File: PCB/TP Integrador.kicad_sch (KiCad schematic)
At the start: 37 parts, among them Q1 BC547C, Q10 BC547C, Q11 BC547C, Q2 2SB631, Q3 BC547, Q4 BC547C, Q5 BC557C, Q6 BC557C, Q9 BC547C, U1 TL431D

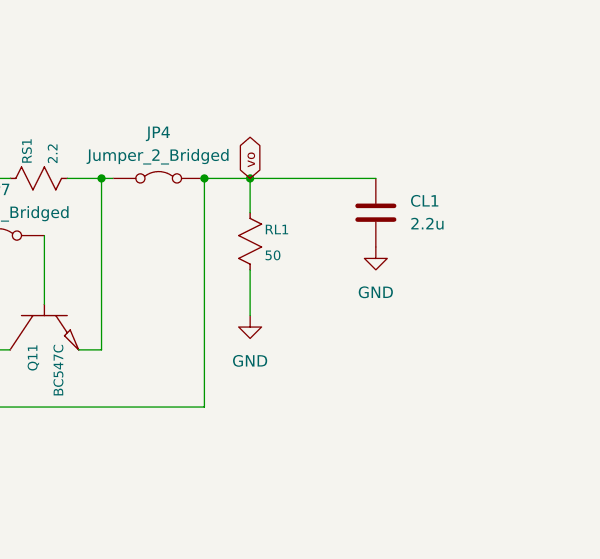
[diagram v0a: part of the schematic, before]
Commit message: Falta el disipador!!!
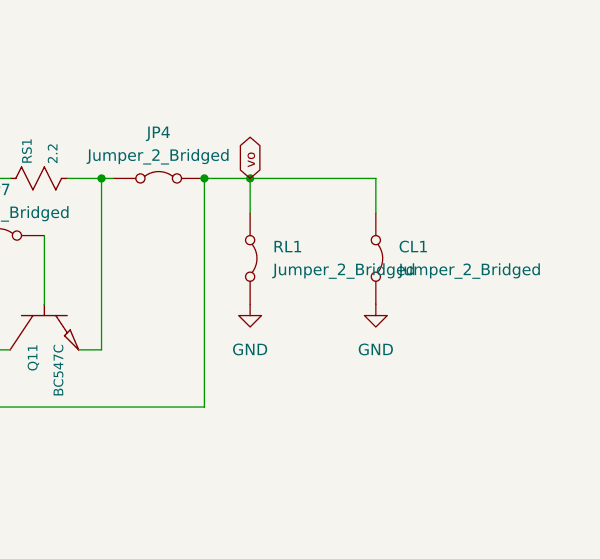
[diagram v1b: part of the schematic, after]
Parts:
- removed CL1: 2.2u, Capacitor_THT:CP_Radial_D8.0mm_P3.80mm, symbol Device:C
- removed RL1: 50, Resistor_THT:R_Axial_DIN0207_L6.3mm_D2.5mm_P7.62mm_Horizontal, symbol ltspice:res
- added CL1, RL1: Jumper_2_Bridged, TestPoint:TestPoint_2Pads_Pitch5.08mm_Drill1.3mm, symbol Jumper:Jumper_2_Bridged
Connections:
- net GND: now also CL1.2 (B), RL1.2 (B)
- net vo: now also CL1.1 (A), RL1.1 (A)
